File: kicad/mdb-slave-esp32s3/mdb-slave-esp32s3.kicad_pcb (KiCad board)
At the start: 2 copper layers, 39 x 40 mm, 45 parts, among them J1 MDB_Connector, J2 USB_C_Receptacle_USB2.0_16P, J3 Conn_01x03_Pin, J8 Conn_01x04_Pin, Q7 MMBT3904, SW1 SW_Push, U1 TLP785, U3 ESP32-S3FH4R2, U4 TLP785, U5 LM2594HVM-3.3, Y1 Crystal_GND24

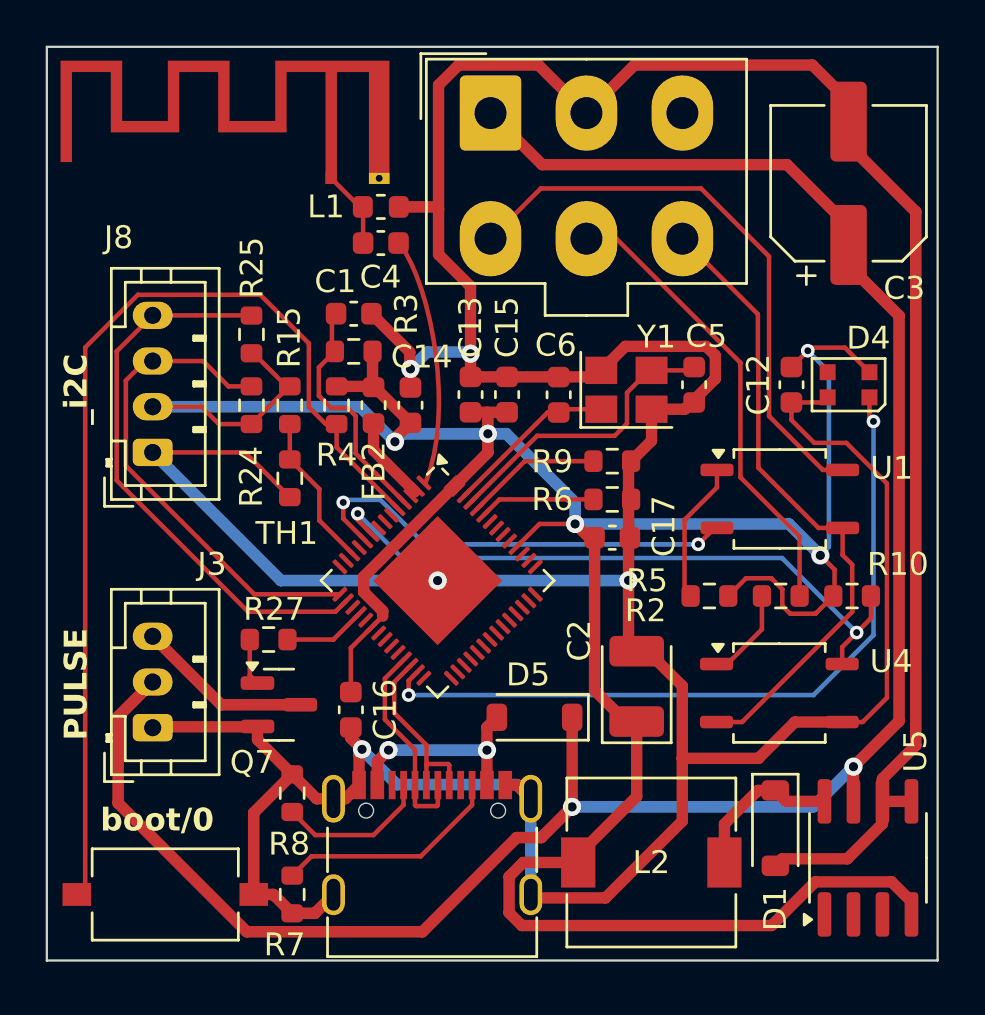
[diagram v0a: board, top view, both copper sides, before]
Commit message: routing...
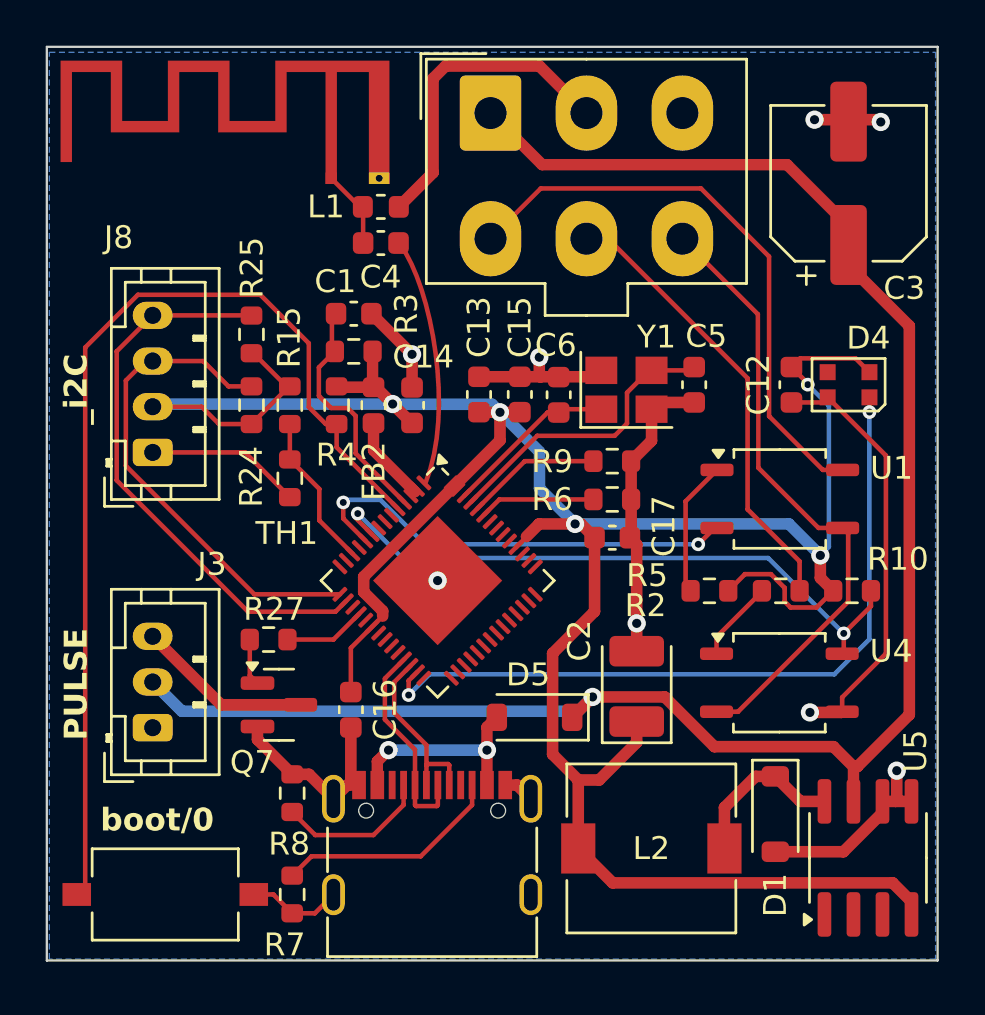
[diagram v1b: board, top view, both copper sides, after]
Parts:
- moved D1 0.61 mm to (200.4, 116.7)
- moved L2 0.61 mm to (195.0, 118.2)
- moved C15 0.56 mm to (189.2, 98.3)
- moved U4 0.45 mm to (200.6, 110.9)
- moved C13 0.37 mm to (187.4, 98.3)
- moved R10 0.23 mm to (203.8, 106.9)
- moved R2 0.23 mm to (200.6, 106.9)
- moved R5 0.23 mm to (197.5, 106.9)
- moved C14 0.07 mm to (184.5, 98.8)
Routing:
- net GND: track 221.3 -> 89.0 mm, vias 5 -> 8
- net /vin: track 92.0 -> 79.1 mm, vias 2 -> 1
- net +3V3: track 132.6 -> 125.3 mm
- net /io4: track 28.8 -> 28.0 mm
- net /mdb_communications_common: track 28.0 -> 27.3 mm
- net Net-(R2-Pad2): track 4.08 -> 3.58 mm
- added copper zone on B.Cu, net GND
